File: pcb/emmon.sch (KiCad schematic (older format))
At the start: 46 parts, among them J1 PROG_CONN, J2 ANT_CONN, J3 AC_CONN, Q1 PT11-21C, U1 DS3231MZ, U2 AT24CS32-SSHM, U3 Ai-Thinker-Ra-01, U4 ESP-12F, U5 LM393

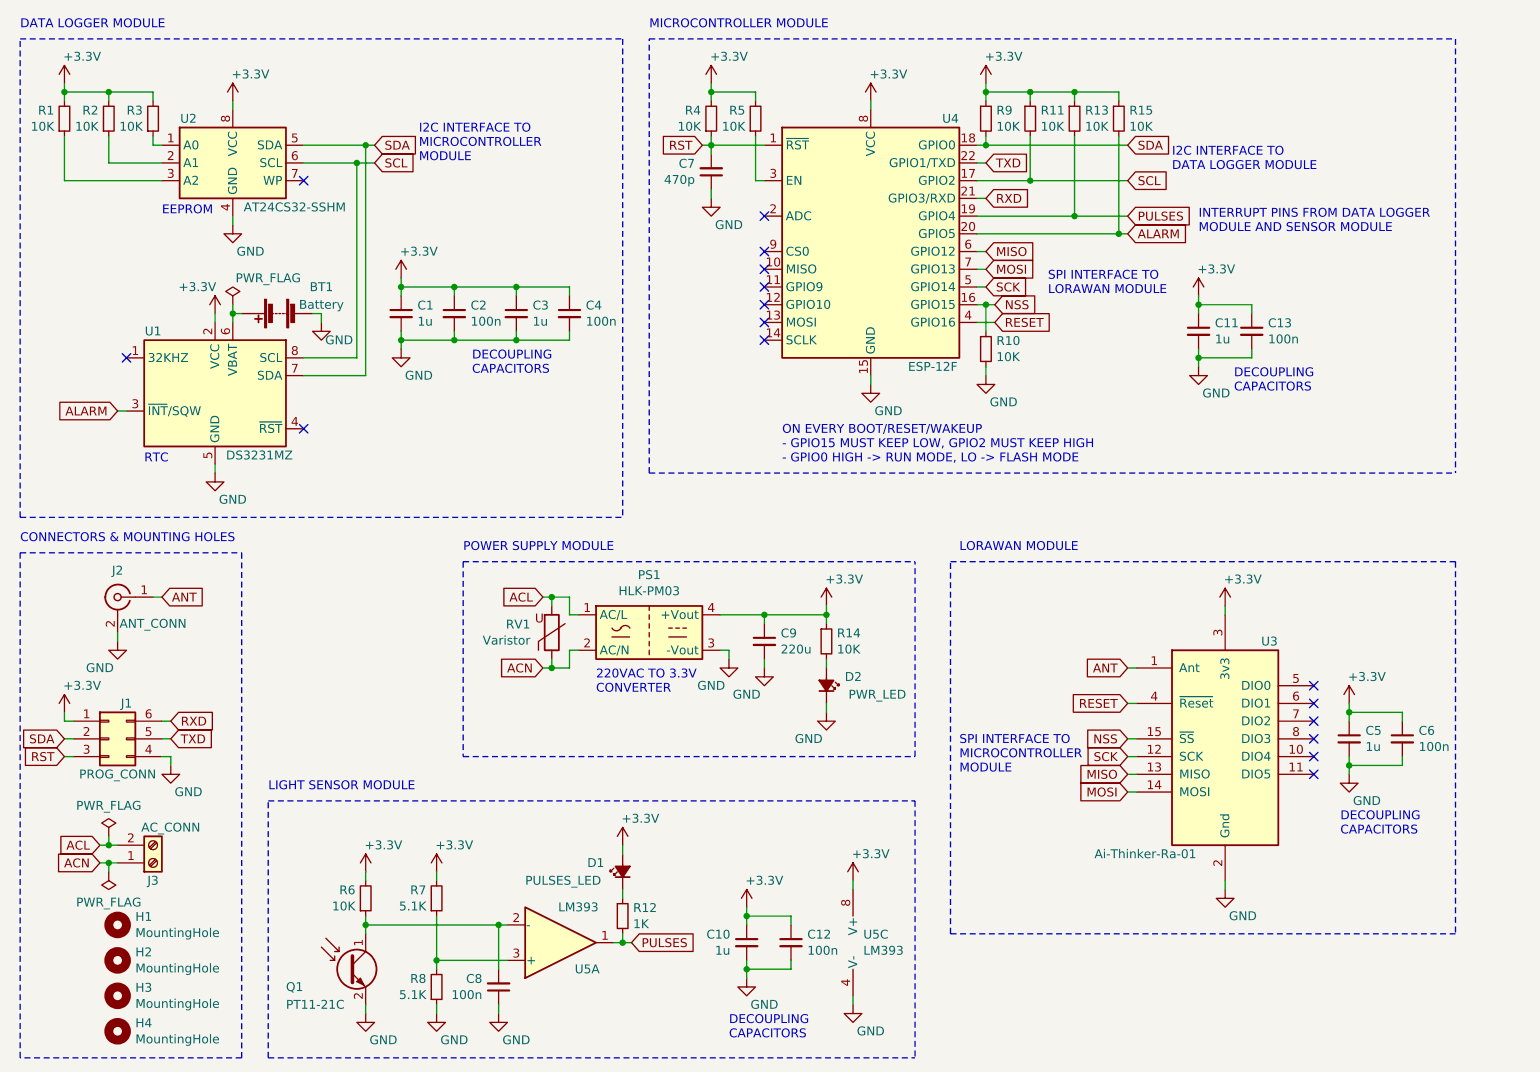
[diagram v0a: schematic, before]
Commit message: Se corrigen las observaciones del docente
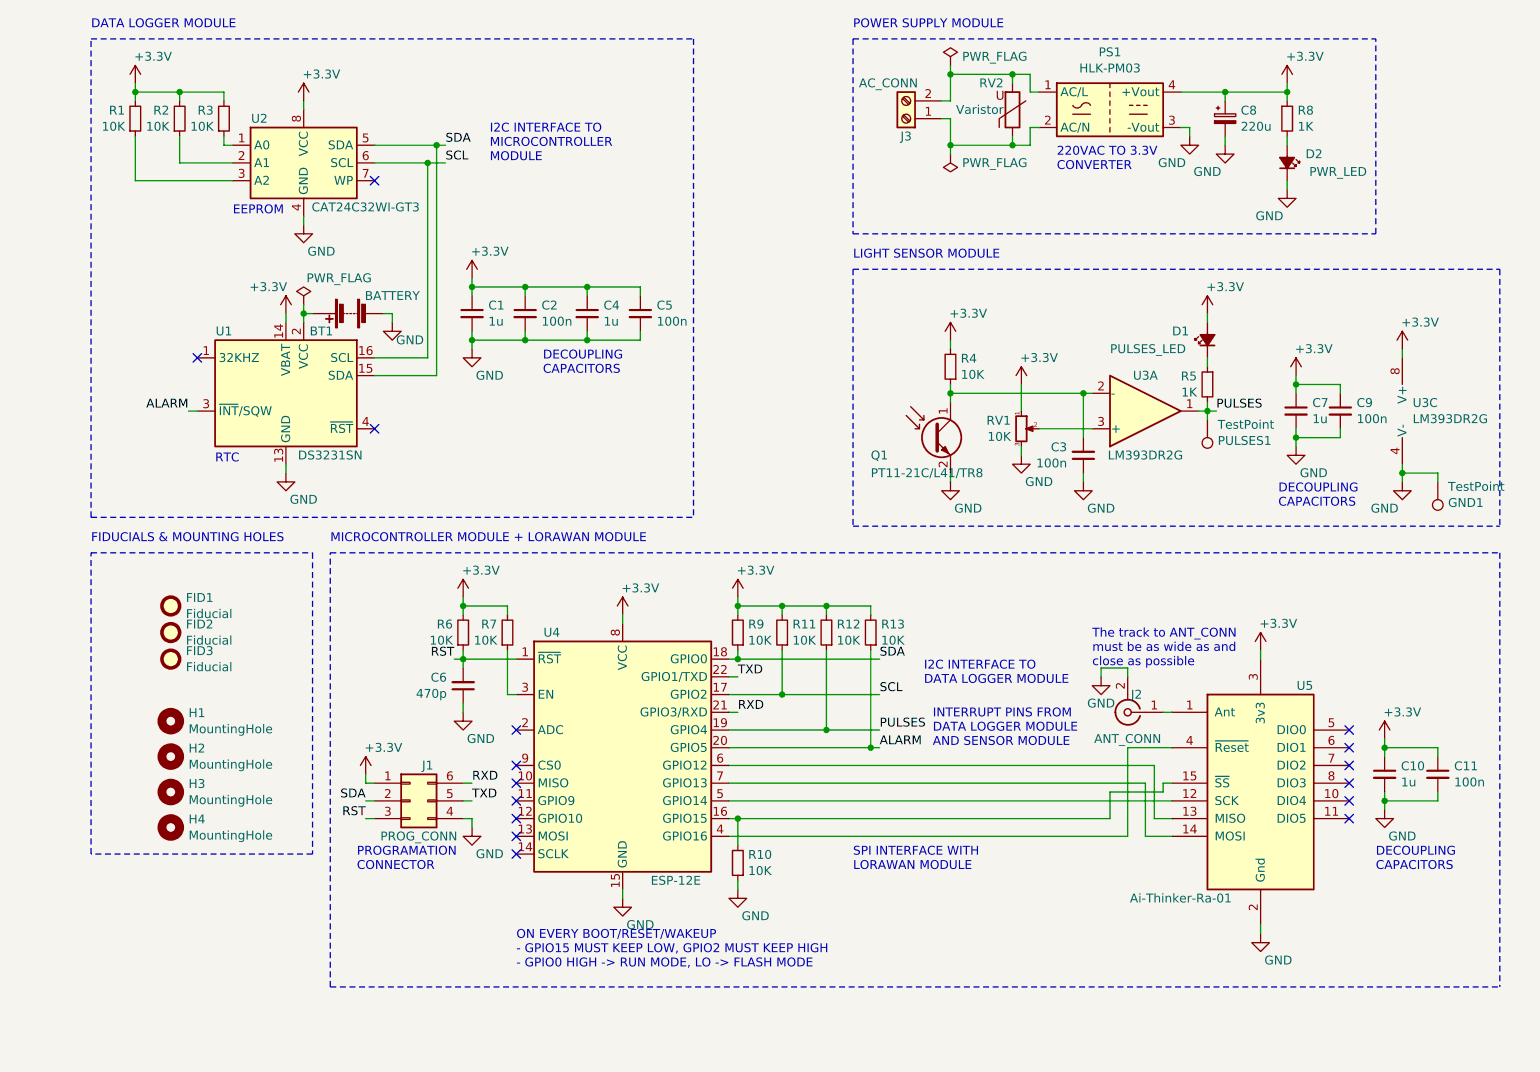
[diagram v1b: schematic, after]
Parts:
- removed C10, C11, C3: 1u, Capacitor_SMD:C_0805_2012Metric_Pad1.15x1.40mm_HandSolder, symbol Device:C_Small
- removed C12, C13: 100n, Capacitor_SMD:C_0805_2012Metric_Pad1.15x1.40mm_HandSolder, symbol Device:C_Small
- removed R14, R15, R5: 10K, Resistor_SMD:R_0805_2012Metric_Pad1.15x1.40mm_HandSolder, symbol Device:R_Small
- removed U1: DS3231MZ, Package_SO:SOIC-8_3.9x4.9mm_P1.27mm, symbol Timer_RTC:DS3231MZ
- removed U4: ESP-12F, RF_Module:ESP-12E, symbol RF_Module:ESP-12F
- added C5: 100n, Capacitor_SMD:C_0805_2012Metric_Pad1.15x1.40mm_HandSolder, symbol Device:C_Small
- added C7: 1u, Capacitor_SMD:C_0805_2012Metric_Pad1.15x1.40mm_HandSolder, symbol Device:C_Small
- added C8: 220u, Capacitor_THT:C_Radial_D6.3mm_H11.0mm_P2.50mm, symbol Device:CP_Small
- added FID1, FID2, FID3: Fiducial, Fiducial:Fiducial_1mm_Mask2mm, symbol Mechanical:Fiducial
- added GND1, PULSES1: TestPoint, TestPoint:TestPoint_THTPad_3.0x3.0mm_Drill1.5mm, symbol Connector:TestPoint
- added R12: 10K, Resistor_SMD:R_0805_2012Metric_Pad1.15x1.40mm_HandSolder, symbol Device:R_Small
- added RV1: 10K, Potentiometer_THT:Potentiometer_Bourns_3386P_Vertical, symbol Device:R_POT_Small
- added U1: DS3231SN, Package_SO:SOIC-16W_7.5x10.3mm_P1.27mm, symbol Timer_RTC:DS3231M
- added U4: ESP-12E, RF_Module:ESP-12E, symbol RF_Module:ESP-12E
- BT1: value Battery -> BATTERY; Description (none) -> SMD Battery Holders, Clips & Contacts RoHS; LCSC (none) -> C70377
- C1: Description (none) -> Multilayer Ceramic Capacitors MLCC - SMD/SMT 1uF 50V 0805 R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; LCSC (none) -> C28323
- C10: renamed from C5; Description (none) -> Multilayer Ceramic Capacitors MLCC - SMD/SMT 1uF 50V 0805 R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; LCSC (none) -> C28323
- C11: renamed from C6; Description (none) -> Multilayer Ceramic Capacitors MLCC - SMD/SMT 100nF 50V 0805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; LCSC (none) -> C49678
- C2: Description (none) -> Multilayer Ceramic Capacitors MLCC - SMD/SMT 100nF 50V 0805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; LCSC (none) -> C49678
- C4: value 100n -> 1u; Description (none) -> Multilayer Ceramic Capacitors MLCC - SMD/SMT 1uF 50V 0805 R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; LCSC (none) -> C28323
- C6: renamed from C7; Description (none) -> Multilayer Ceramic Capacitors MLCC - SMD/SMT 470pF 50V 0805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; LCSC (none) -> C1743
- C9: value 220u -> 100n; footprint Capacitor_THT:C_Radial_D6.3mm_H11.0mm_P2.50mm -> Capacitor_SMD:C_0805_2012Metric_Pad1.15x1.40mm_HandSolder; Description (none) -> Multilayer Ceramic Capacitors MLCC - SMD/SMT 100nF 50V 0805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; LCSC (none) -> C49678
- J1: Description (none) -> Pin Header Male Pin 0.100\"(2.54mm) 6 2 P=2.54mm Pin Header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; LCSC (none) -> C65114
- J2: Description (none) -> RF Connectors/Coaxial Connectors RoHS; LCSC (none) -> C496550
- J3: Description (none) -> P=5.08mm Screw terminal RoHS; LCSC (none) -> C89120
- PS1: Description (none) -> Through Hole Power Module AC-DC RoHS; LCSC (none) -> C209904
- Q1: value PT11-21C -> PT11-21C/L41/TR8; Description (none) -> 20mA 100nA 940nm 400nm-1100nm 30V 1206 Infrared Receivers R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; LCSC (none) -> C16746
- R1, R10, R11, R13, R2, R3, R4, R6, R9: Description (none) -> Chip Resistor - Surface Mount 10KOhms ±1% 1/8W 0805 RoHS; LCSC (none) -> C17414
- R5: renamed from R12; Description (none) -> Chip Resistor - Surface Mount 1KOhms ±1% 1/8W 0805 RoHS; LCSC (none) -> C17513
- R7: value 5.1K -> 10K; Description (none) -> Chip Resistor - Surface Mount 10KOhms ±1% 1/8W 0805 RoHS; LCSC (none) -> C17414
- R8: value 5.1K -> 1K; Description (none) -> Chip Resistor - Surface Mount 1KOhms ±1% 1/8W 0805 RoHS; LCSC (none) -> C17513
- RV2: renamed from RV1; Description (none) -> 460V 925V 2.5KA 560V Through Hole Varistors RoHS; LCSC (none) -> C233178
- U2: value AT24CS32-SSHM -> CAT24C32WI-GT3; Description (none) -> EEPROM EEPROM 32Kb (4K x 8) I2C SOIC-8_150mil RoHS; LCSC (none) -> C81193
- U3: renamed from U5; value LM393 -> LM393DR2G; Description (none) -> Analog Comparators 2V - 36V, ±1V ~ 18V SOIC-8_150mil RoHS; LCSC (none) -> C7955
- U3: renamed from U5; value LM393 -> LM393DR2G
- U5: renamed from U3; Description (none) -> Wireless Modules RoHS; LCSC (none) -> C90040
- renumbered C8 to C3
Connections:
- net +3V3: now also R11.2, R13.2, R8.1, R9.2, C5.1, C7.1, C8.1, R12.2, RV1.1, U1.14 (VBAT), U4.8 (VCC); no longer R11.1, R13.1, R9.1
- net ALARM: now also R13.1, U1.3 (~INT~/SQW), U4.20 (GPIO5)
- net GND: now also R10.1, C5.2, C7.2, C8.2, GND1.1, RV1.3, U1.10 (GND), U1.11 (GND), U1.12 (GND), U1.13 (GND), U1.5 (GND), U1.6 (GND), U1.7 (GND), U1.8 (GND), U1.9 (GND), U4.15 (GND); no longer R10.2, R8.1
- net PULSES: now also PULSES1.1, R12.1, U4.19 (GPIO4); no longer R13.2
- net RST: now also R6.1, U4.1 (~RST); no longer R4.1
- net RXD: now also U4.21 (GPIO3/RXD)
- net SCL: now also R11.1, U1.16 (SCL), U4.17 (GPIO2); no longer R11.2
- net SDA: now also R9.1, U1.15 (SDA), U4.18 (GPIO0); no longer R9.2
- net TXD: now also U4.22 (GPIO1/TXD)
- net at BT1.1 (+): now also U1.2 (VCC)
- net at C3.2, Q1.1 (C), U3.2 (-): now also R4.1; no longer R6.1
- net at D2.2 (A): now also R8.2
- net ACL: no longer names the net of J3.2 (Pin_2), PS1.1 (AC/L), RV2.2
- net ACN: no longer names the net of J3.1 (Pin_1), PS1.2 (AC/N), RV2.1
- net ANT: no longer names the net of J2.1 (In), U5.1 (Ant)
- net MISO: no longer names the net of U5.13 (MISO)
- net MISO: now also U4.6 (GPIO12)
- net MOSI: no longer names the net of U5.14 (MOSI)
- net MOSI: now also U4.7 (GPIO13)
- net NSS: no longer names the net of U5.15 (~SS)
- net NSS: now also R10.2, U4.16 (GPIO15); no longer R10.1
- net RESET: no longer names the net of U5.4 (~Reset)
- net RESET: now also U4.4 (GPIO16)
- net SCK: no longer names the net of U5.12 (SCK)
- net SCK: now also U4.5 (GPIO14)
- new net: RV1.2, U3.3 (+)
- new net: R7.1, U4.3 (EN)
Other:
- note added: "FIDUCIALS & MOUNTING HOLES"
- note added: "INTERRUPT PINS FROM\nDATA LOGGER MODULE \nAND SENSOR MODULE"
- note added: "MICROCONTROLLER MODULE + LORAWAN MODULE"
- note added: "PROGRAMATION\nCONNECTOR"
- note added: "SPI INTERFACE WITH\nLORAWAN MODULE"
- note added: "The track to ANT_CONN\nmust be as wide as and \nclose as possible"
- note removed: "CONNECTORS & MOUNTING HOLES"
- note removed: "INTERRUPT PINS FROM DATA LOGGER\nMODULE AND SENSOR MODULE"
- note removed: "LORAWAN MODULE"
- note removed: "MICROCONTROLLER MODULE"
- note removed: "SPI INTERFACE TO \nLORAWAN MODULE"
- note removed: "SPI INTERFACE TO \nMICROCONTROLLER\nMODULE"
- moved on the sheet: BT1, C10, C11, C3, C6, D1, D2, H1, H2, H3, H4, J1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
